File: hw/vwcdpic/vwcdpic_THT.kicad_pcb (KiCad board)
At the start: 2 copper layers, 30.6 x 16.4 mm, 11 parts, among them U1 PIC12F629, U2 LM78L05ACZ

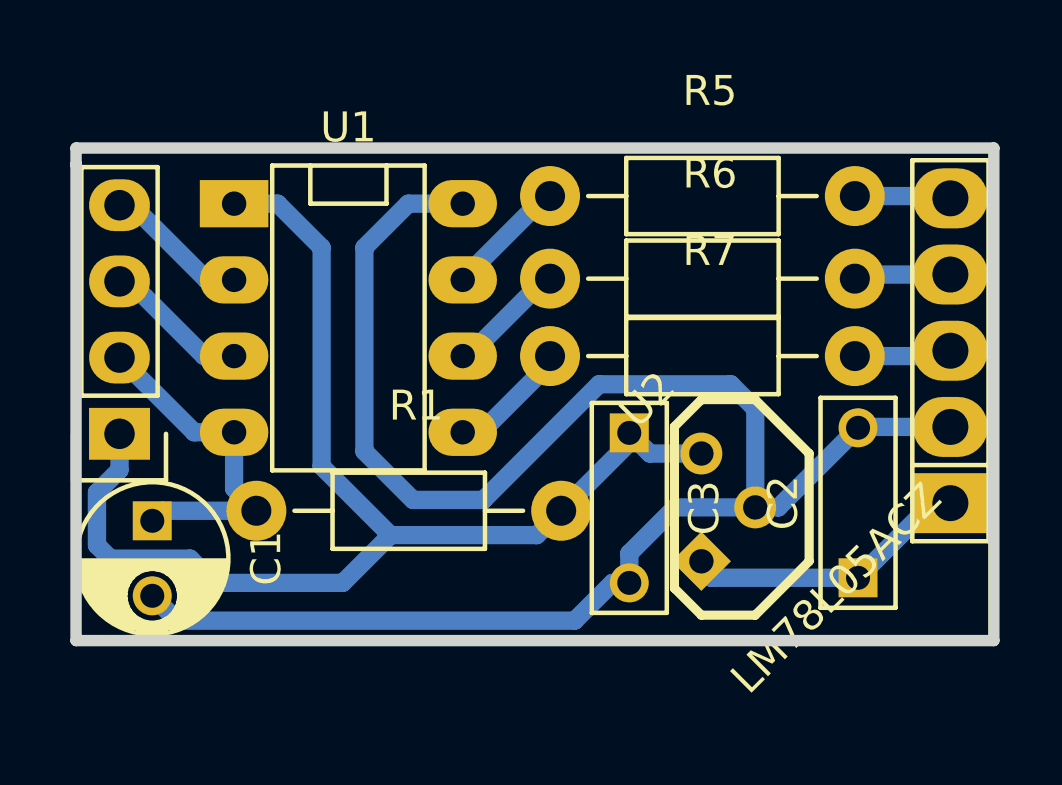
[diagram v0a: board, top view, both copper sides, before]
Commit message: update, new schematics file
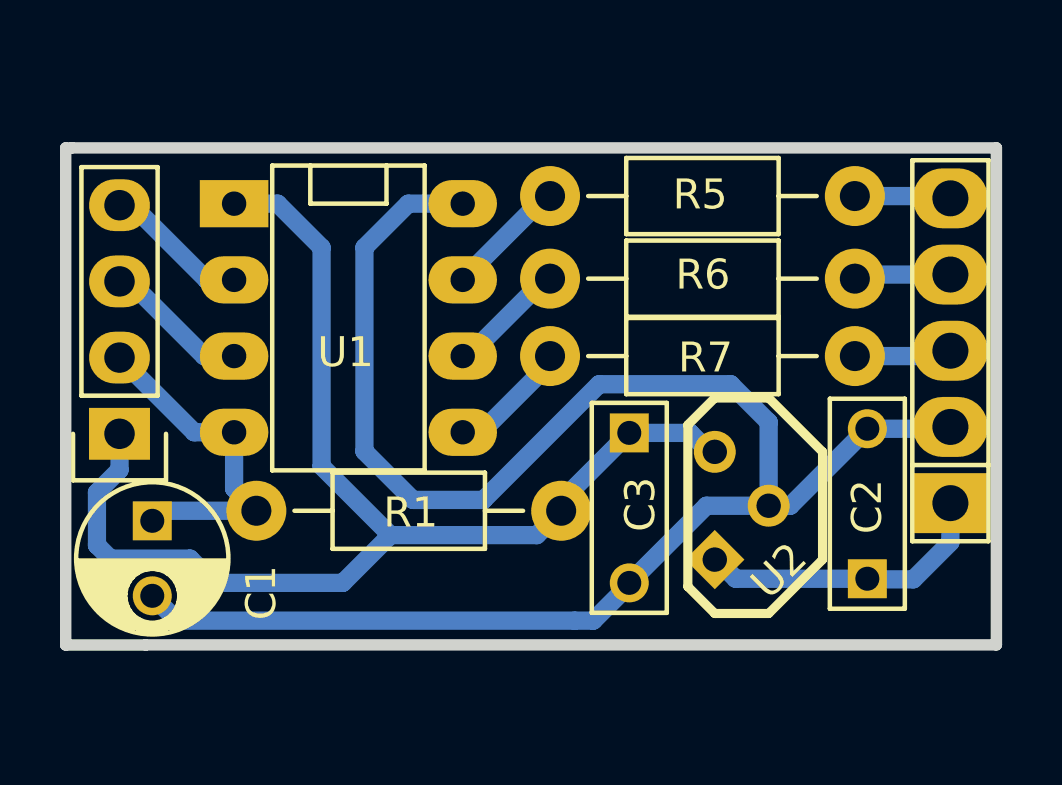
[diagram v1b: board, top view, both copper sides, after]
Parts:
- moved U2 0.45 mm to (151.6, 139.1)
- moved C2 0.31 mm to (156.7, 141.6)
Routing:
- net +5V: track 41.4 -> 42.2 mm
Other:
- board size 30.6 x 16.4 mm -> 31 x 16.6 mm
